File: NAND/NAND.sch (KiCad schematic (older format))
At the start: 2 parts

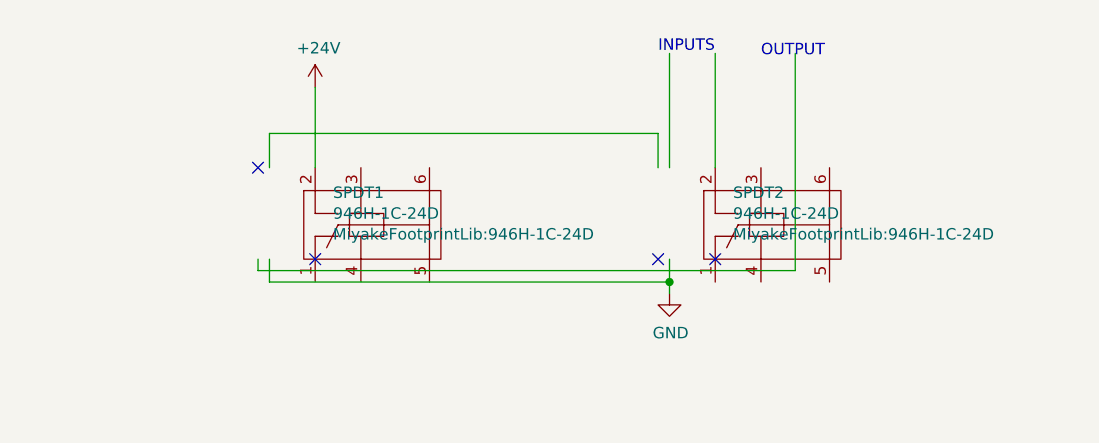
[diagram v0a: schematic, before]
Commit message: Add files via upload
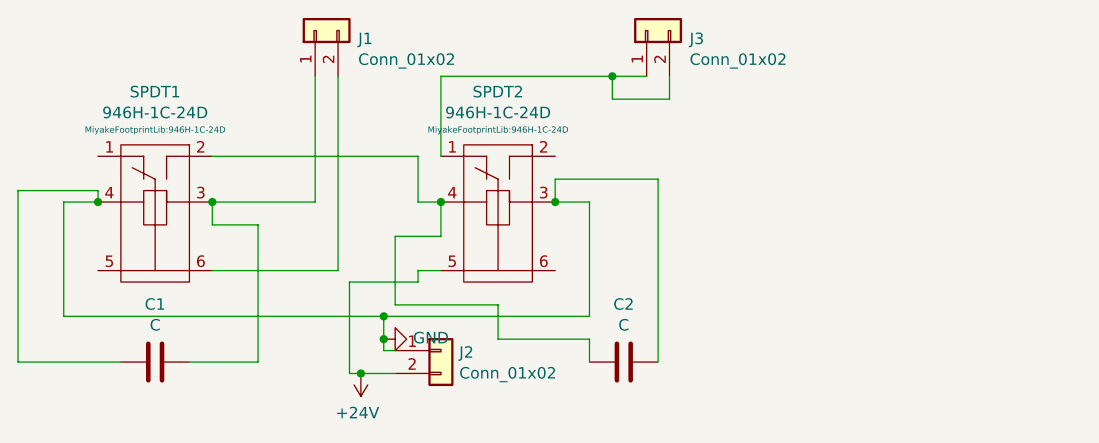
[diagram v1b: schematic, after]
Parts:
- added C1, C2: C, MiyakeFootprintLib:Condensor, symbol Device:C
- added J1, J2, J3: Conn_01x02, Connector_PinHeader_2.54mm:PinHeader_1x02_P2.54mm_Vertical, symbol Connector_Generic:Conn_01x02
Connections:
- wire segments 13 -> 46
- no-connect marks 4 -> 0
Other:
- note removed: "INPUTS"
- note removed: "OUTPUT\n\n"
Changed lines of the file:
@@
 $Comp
 L MiyakeLib:946H-1C-24D SPDT1
-U 1 1 5ED35ECC
-P 4400 3000
-F 0 "SPDT1" V 4491 2772 50  0000 R CNN
-F 1 "946H-1C-24D" V 4400 2772 50  0000 R CNN
-F 2 "MiyakeFootprintLib:946H-1C-24D" V 4309 2772 50  0000 R CNN
-F 3 "" H 4350 3250 50  0001 C CNN
-	1    4400 3000
+U 1 1 5ED8B7A7
+P 3900 2600
+F 0 "SPDT1" H 3850 2731 50  0000 C CNN
+F 1 "946H-1C-24D" H 3850 2640 50  0000 C CNN
+F 2 "MiyakeFootprintLib:946H-1C-24D" H 3850 2566 27  0000 C CNN
+F 3 "" V 3850 2050 50  0001 C CNN
+	1    3900 2600
+	1    0    0    -1
+$EndComp
+$Comp
+L MiyakeLib:946H-1C-24D SPDT2
+U 1 1 5ED8BE6F
+P 5400 2600
+F 0 "SPDT2" H 5350 2731 50  0000 C CNN
+F 1 "946H-1C-24D" H 5350 2640 50  0000 C CNN
+F 2 "MiyakeFootprintLib:946H-1C-24D" H 5350 2566 27  0000 C CNN
+F 3 "" V 5350 2050 50  0001 C CNN
+	1    5400 2600
+	1    0    0    -1
+$EndComp
+$Comp
+L Connector_Generic:Conn_01x02 J1
+U 1 1 5ED8DDA6
+P 4550 2200
+F 0 "J1" V 4514 2012 50  0000 R CNN
+F 1 "Conn_01x02" V 4423 2012 50  0000 R CNN
+F 2 "Connector_PinHeader_2.54mm:PinHeader_1x02_P2.54mm_Vertical" H 4550 2200 50  0001 C CNN
+F 3 "~" H 4550 2200 50  0001 C CNN
+	1    4550 2200
 	0    -1   -1   0
 $EndComp
-$Comp
-L MiyakeLib:946H-1C-24D SPDT2
-U 1 1 5ED3673F
-P 6150 3000
-F 0 "SPDT2" V 6241 2772 50  0000 R CNN
-F 1 "946H-1C-24D" V 6150 2772 50  0000 R CNN
-F 2 "MiyakeFootprintLib:946H-1C-24D" V 6059 2772 50  0000 R CNN
-F 3 "" H 6100 3250 50  0001 C CNN
-	1    6150 3000
+Wire Wire Line
+	4550 2400 4550 2950
+Wire Wire Line
+	4550 2950 4100 2950
+$Comp
+L Connector_Generic:Conn_01x02 J3
+U 1 1 5ED8EE55
+P 6000 2200
+F 0 "J3" V 5964 2012 50  0000 R CNN
+F 1 "Conn_01x02" V 5873 2012 50  0000 R CNN
+F 2 "Connector_PinHeader_2.54mm:PinHeader_1x02_P2.54mm_Vertical" H 6000 2200 50  0001 C CNN
+F 3 "~" H 6000 2200 50  0001 C CNN
+	1    6000 2200
 	0    -1   -1   0
 $EndComp
-Wire Wire Line
-	6100 2800 6100 2300
-Wire Wire Line
-	6300 2800 6300 2300
-Wire Wire Line
-	6050 2800 6050 2650
-Wire Wire Line
-	6050 2650 4350 2650
-Wire Wire Line
-	4350 2650 4350 2800
-Wire Wire Line
-	6100 3200 6100 3300
-Wire Wire Line
-	6100 3300 4350 3300
-Wire Wire Line
-	4350 3300 4350 3200
-Connection ~ 6100 3300
-Wire Wire Line
-	6100 3300 6100 3350
-Wire Wire Line
-	4300 3200 4300 3250
-Wire Wire Line
-	4300 3250 6650 3250
-Wire Wire Line
-	6650 3250 6650 2300
-Wire Wire Line
-	4550 2800 4550 2450
-$Comp
-L power:+24V #PWR01
-U 1 1 5ED3830F
-P 4550 2450
-F 0 "#PWR01" H 4550 2300 50  0001 C CNN
-F 1 "+24V" H 4565 2623 50  0000 C CNN
-F 2 "" H 4550 2450 50  0001 C CNN
-F 3 "" H 4550 2450 50  0001 C CNN
-	1    4550 2450
+$Comp
+L Connector_Generic:Conn_01x02 J2
+U 1 1 5ED8FB42
+P 5100 3600
+F 0 "J2" H 5180 3592 50  0000 L CNN
+F 1 "Conn_01x02" H 5180 3501 50  0000 L CNN
+F 2 "Connector_PinHeader_2.54mm:PinHeader_1x02_P2.54mm_Vertical" H 5100 3600 50  0001 C CNN
+F 3 "~" H 5100 3600 50  0001 C CNN
+	1    5100 3600
 	1    0    0    -1
 $EndComp
-$Comp
-L power:GND #PWR02
-U 1 1 5ED3873E
-P 6100 3350
-F 0 "#PWR02" H 6100 3100 50  0001 C CNN
-F 1 "GND" H 6105 3177 50  0000 C CNN
-F 2 "" H 6100 3350 50  0001 C CNN
-F 3 "" H 6100 3350 50  0001 C CNN
-	1    6100 3350
-	1    0    0    -1
-$EndComp
-Text Notes 6050 2300 0    50   ~ 0
-INPUTS
-Text Notes 6500 2400 0    50   ~ 0
-OUTPUT\n\n
-NoConn ~ 6050 3200
-NoConn ~ 6300 3200
-NoConn ~ 4550 3200
-NoConn ~ 4300 2800
+Wire Wire Line
+	3600 2950 3450 2950
+Wire Wire Line
+	3450 2950 3450 3450
+Wire Wire Line
+	3450 3450 4850 3450
+Wire Wire Line
+	5750 3450 5750 2950
+Wire Wire Line
+	5750 2950 5600 2950
+Wire Wire Line
+	4850 3450 4850 3550
+Wire Wire Line
+	4850 3600 4900 3600
+Connection ~ 4850 3450
+Wire Wire Line
+	4850 3450 5750 3450
+Wire Wire Line
+	4650 2400 4650 3250
+Wire Wire Line
+	4650 3250 4100 3250
+Wire Wire Line
+	4100 2750 5000 2750
+Wire Wire Line
+	5000 2750 5000 2950
+Wire Wire Line
+	5000 2950 5100 2950
+Wire Wire Line
+	4900 3700 4750 3700
+Wire Wire Line
+	4700 3700 4700 3300
+Wire Wire Line
+	4700 3300 5000 3300
+Wire Wire Line
+	5000 3300 5000 3250
+Wire Wire Line
+	5000 3250 5100 3250
+Wire Wire Line
+	5100 2750 5100 2400
+Wire Wire Line
+	5100 2400 5850 2400
+Wire Wire Line
+	5850 2400 5850 2500
+Wire Wire Line
+	5850 2500 6100 2500
+Wire Wire Line
+	6100 2500 6100 2400
+Connection ~ 5850 2400
+Wire Wire Line
+	5850 2400 6000 2400
+$Comp
+L Device:C C2
+U 1 1 5ED9244B
+P 5900 3650
+F 0 "C2" V 5648 3650 50  0000 C CNN
+F 1 "C" V 5739 3650 50  0000 C CNN
+F 2 "MiyakeFootprintLib:Condensor" H 5938 3500 50  0001 C CNN
+F 3 "~" H 5900 3650 50  0001 C CNN
+	1    5900 3650
+	0    1    1    0
+$EndComp
+$Comp
+L Device:C C1
+U 1 1 5ED92B44
+P 3850 3650
+F 0 "C1" V 3598 3650 50  0000 C CNN
+F 1 "C" V 3689 3650 50  0000 C CNN
+F 2 "MiyakeFootprintLib:Condensor" H 3888 3500 50  0001 C CNN
+F 3 "~" H 3850 3650 50  0001 C CNN
+	1    3850 3650
+	0    1    1    0
+$EndComp
+Wire Wire Line
+	6050 3650 6050 2850
+Wire Wire Line
+	6050 2850 5600 2850
+Wire Wire Line
+	5600 2850 5600 2950
+Connection ~ 5600 2950
+Wire Wire Line
+	5750 3650 5750 3550
+Wire Wire Line
+	5750 3550 5350 3550
+Wire Wire Line
+	5350 3550 5350 3400
+Wire Wire Line
+	4900 3400 4900 3100
+Wire Wire Line
+	4900 3100 5100 3100
+Wire Wire Line
+	5100 3100 5100 2950
+Wire Wire Line
+	4900 3400 5350 3400
+Connection ~ 5100 2950
+Wire Wire Line
+	4000 3650 4300 3650
+Wire Wire Line
+	4300 3650 4300 3050
+Wire Wire Line
+	4300 3050 4100 3050
+Wire Wire Line
+	4100 3050 4100 2950
+Connection ~ 4100 2950
+Wire Wire Line
+	3700 3650 3250 3650
+Wire Wire Line
+	3250 3650 3250 2900
+Wire Wire Line
+	3250 2900 3600 2900
+Wire Wire Line
+	3600 2900 3600 2950
+Connection ~ 3600 2950
+$Comp
+L power:GND #PWR?
+U 1 1 5ED9602B
+P 4850 3550
+F 0 "#PWR?" H 4850 3300 50  0001 C CNN
+F 1 "GND" V 4855 3422 50  0000 R CNN
+F 2 "" H 4850 3550 50  0001 C CNN
+F 3 "" H 4850 3550 50  0001 C CNN
+	1    4850 3550
+	0    -1   -1   0
+$EndComp
+Connection ~ 4850 3550
+Wire Wire Line
+	4850 3550 4850 3600
+$Comp
+L power:+24V #PWR?
+U 1 1 5ED9653B
+P 4750 3700
+F 0 "#PWR?" H 4750 3550 50  0001 C CNN
+F 1 "+24V" H 4765 3873 50  0000 C CNN
+F 2 "" H 4750 3700 50  0001 C CNN
+F 3 "" H 4750 3700 50  0001 C CNN
+	1    4750 3700
+	-1   0    0    1
+$EndComp
+Connection ~ 4750 3700
+Wire Wire Line
+	4750 3700 4700 3700
 $EndSCHEMATC
